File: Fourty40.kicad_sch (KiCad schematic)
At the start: 90 parts, among them SW1 SW_SPST, U1 ProMicro

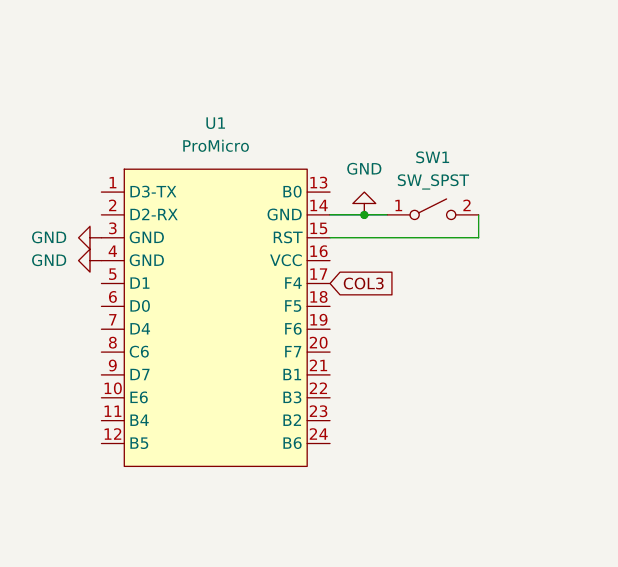
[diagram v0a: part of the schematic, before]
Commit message: PCB update
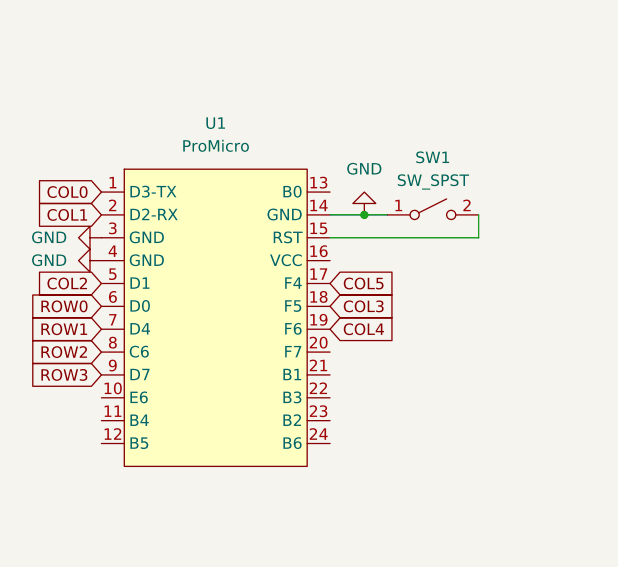
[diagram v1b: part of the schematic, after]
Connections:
- net COL0: now also U1.1 (D3-TX)
- net COL1: now also U1.2 (D2-RX)
- net COL2: now also U1.5 (D1)
- net COL3: now also U1.18 (F5); no longer U1.17 (F4)
- net COL4: now also U1.19 (F6)
- net COL5: now also U1.17 (F4)
- net ROW0: now also U1.6 (D0)
- net ROW1: now also U1.7 (D4)
- net ROW2: now also U1.8 (C6)
- net ROW3: now also U1.9 (D7)
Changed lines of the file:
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@@
+    )
+  )
+  (global_label "ROW1" (shape input) (at 31.75 101.6 180) (fields_autoplaced)
+    (effects (font (size 1.27 1.27)) (justify right))
+    (property "Intersheetrefs" "${INTERSHEET_REFS}" (at 23.5828 101.6 0)
+      (effects (font (size 1.27 1.27)) (justify right) hide)
     )
   )
@@
     )
   )
-  (global_label "COL3" (shape input) (at 57.15 96.52 0) (fields_autoplaced)
+  (global_label "COL4" (shape input) (at 57.15 101.6 0) (fields_autoplaced)
     (effects (font (size 1.27 1.27)) (justify left))
-    (property "Intersheetrefs" "${INTERSHEET_REFS}" (at 64.8939 96.52 0)
+    (property "Intersheetrefs" "${INTERSHEET_REFS}" (at 64.8939 101.6 0)
+      (effects (font (size 1.27 1.27)) (justify left) hide)
+    )
+  )
+  (global_label "COL3" (shape input) (at 57.15 99.06 0) (fields_autoplaced)
+    (effects (font (size 1.27 1.27)) (justify left))
+    (property "Intersheetrefs" "${INTERSHEET_REFS}" (at 64.8939 99.06 0)
       (effects (font (size 1.27 1.27)) (justify left) hide)
     )
@@
     (effects (font (size 1.27 1.27)) (justify right))
     (property "Intersheetrefs" "${INTERSHEET_REFS}" (at 98.5128 143.51 0)
+      (effects (font (size 1.27 1.27)) (justify right) hide)
+    )
+  )
+  (global_label "ROW3" (shape input) (at 31.75 106.68 180) (fields_autoplaced)
+    (effects (font (size 1.27 1.27)) (justify right))
+    (property "Intersheetrefs" "${INTERSHEET_REFS}" (at 23.5828 106.68 0)
+      (effects (font (size 1.27 1.27)) (justify right) hide)
+    )
+  )
+  (global_label "COL0" (shape input) (at 31.75 86.36 180) (fields_autoplaced)
+    (effects (font (size 1.27 1.27)) (justify right))
+    (property "Intersheetrefs" "${INTERSHEET_REFS}" (at 24.0061 86.36 0)
+      (effects (font (size 1.27 1.27)) (justify right) hide)
+    )
+  )
+  (global_label "COL2" (shape input) (at 31.75 96.52 180) (fields_autoplaced)
+    (effects (font (size 1.27 1.27)) (justify right))
+    (property "Intersheetrefs" "${INTERSHEET_REFS}" (at 24.0061 96.52 0)
       (effects (font (size 1.27 1.27)) (justify right) hide)
     )
@@
     )
   )
+  (global_label "ROW2" (shape input) (at 31.75 104.14 180) (fields_autoplaced)
+    (effects (font (size 1.27 1.27)) (justify right))
+    (property "Intersheetrefs" "${INTERSHEET_REFS}" (at 23.5828 104.14 0)
+      (effects (font (size 1.27 1.27)) (justify right) hide)
+    )
+  )
   (global_label "COL2" (shape input) (at 180.34 35.56 90) (fields_autoplaced)
     (effects (font (size 1.27 1.27)) (justify left))
     (property "Intersheetrefs" "${INTERSHEET_REFS}" (at 180.34 27.8161 90)
       (effects (font (size 1.27 1.27)) (justify left) hide)
+    )
+  )
+  (global_label "COL1" (shape input) (at 31.75 88.9 180) (fields_autoplaced)
+    (effects (font (size 1.27 1.27)) (justify right))
+    (property "Intersheetrefs" "${INTERSHEET_REFS}" (at 24.0061 88.9 0)
+      (effects (font (size 1.27 1.27)) (justify right) hide)
     )
   )
@@
       (effects (font (size 1.27 1.27)) (justify left) hide)
     )
+  )
+  (global_label "ROW0" (shape input) (at 31.75 99.06 180) (fields_autoplaced)
+    (effects (font (size 1.27 1.27)) (justify right))
+    (property "Intersheetrefs" "${INTERSHEET_REFS}" (at 23.5828 99.06 0)
+      (effects (font (size 1.27 1.27)) (justify right) hide)
+    )
+  )
+  (global_label "COL5" (shape input) (at 57.15 96.52 0) (fields_autoplaced)
+    (effects (font (size 1.27 1.27)) (justify left))
+    (property "Intersheetrefs" "${INTERSHEET_REFS}" (at 64.8939 96.52 0)
+      (effects (font (size 1.27 1.27)) (justify left) hide)
+    )
